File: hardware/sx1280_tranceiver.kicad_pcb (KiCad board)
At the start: 2 copper layers, 22 parts, among them J1 U.FL-R-SMT-1(80), J2 Conn_02x06_Odd_Even, U1 sx1280, U2 2450FM07D0034, Y1 ECS-520-12-37B-CTN-TR

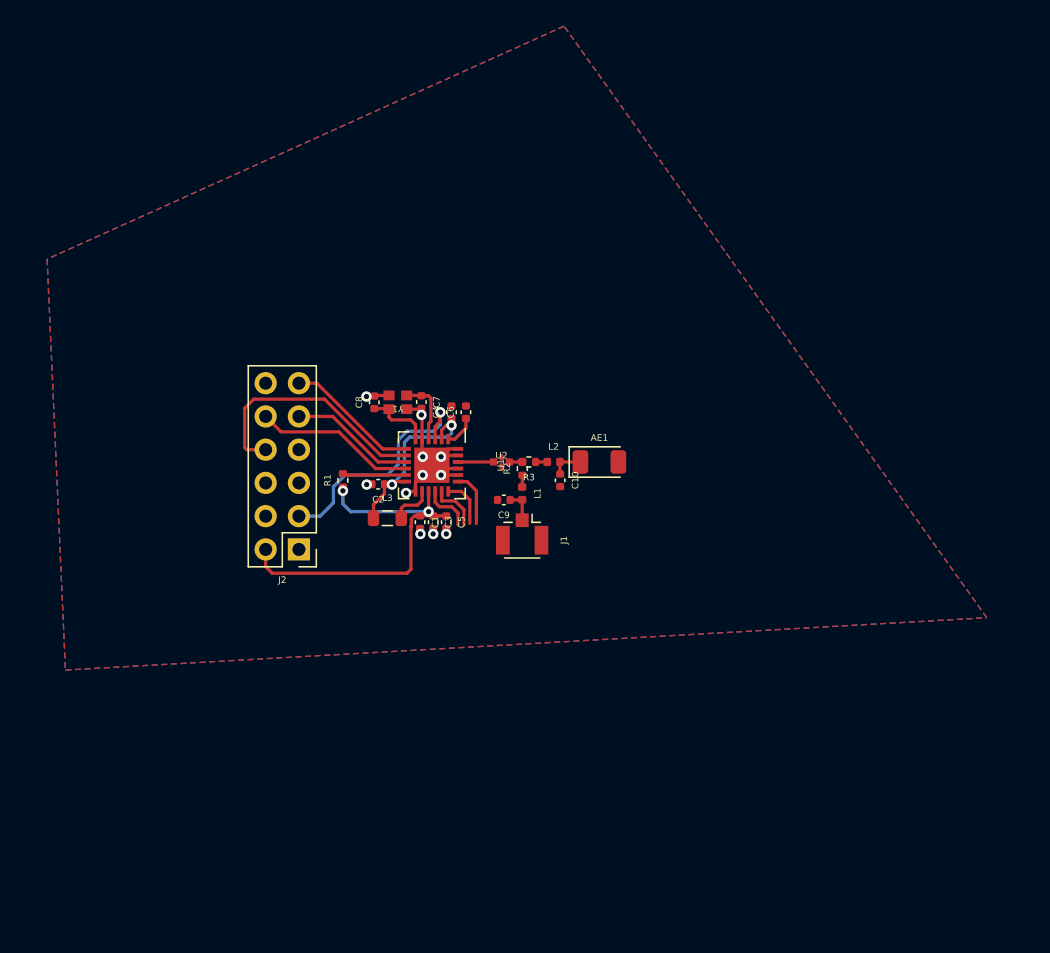
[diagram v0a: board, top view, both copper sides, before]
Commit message: finalized layout
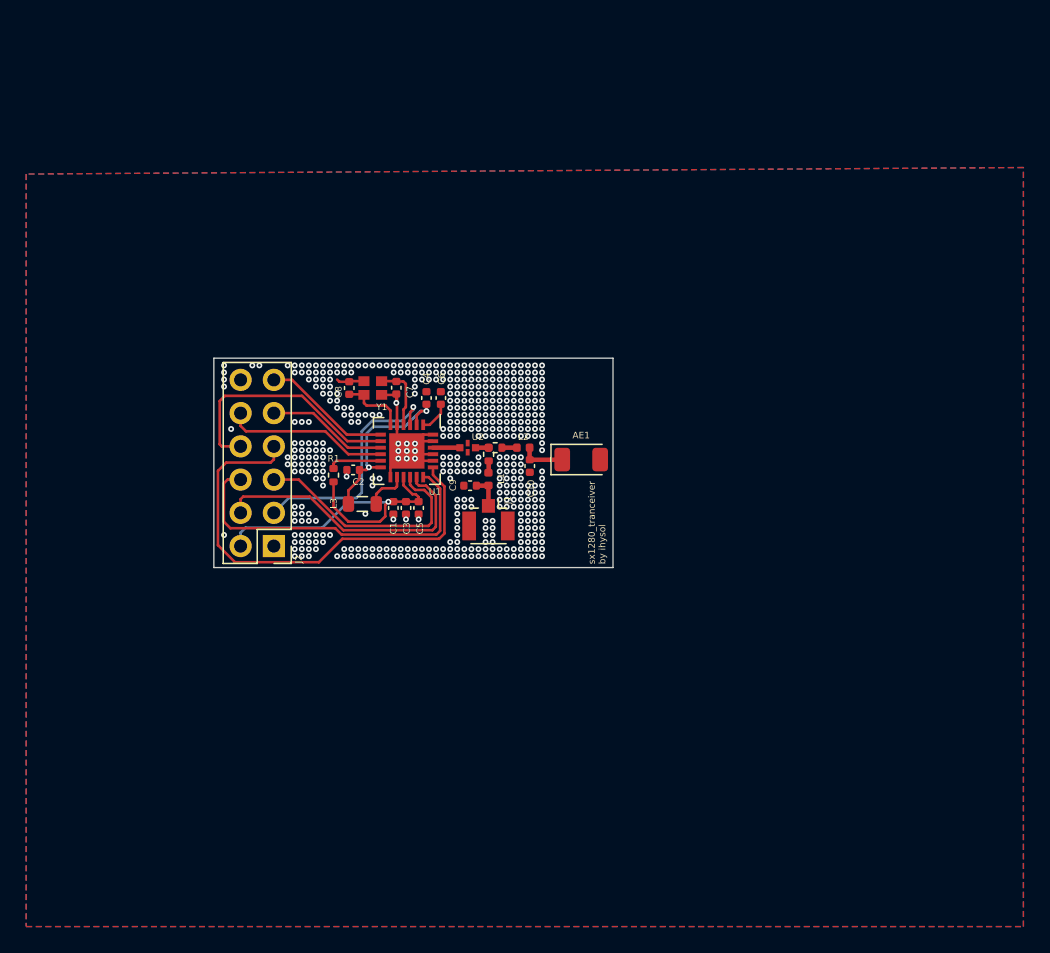
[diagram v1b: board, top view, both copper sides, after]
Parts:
- moved C9 2.80 mm to (84.7, 67.9)
- moved J1 2.80 mm to (86.1, 70.5)
- moved L1 2.80 mm to (86.1, 67.4)
- moved R2 2.80 mm to (86.1, 65.5)
- moved R3 2.80 mm to (86.6, 65.0)
- moved U2 2.80 mm to (84.5, 65.0)
- moved C10 2.56 mm to (89.3, 66.4)
- moved L2 2.56 mm to (88.8, 65.0)
- moved C5 2.38 mm to (80.8, 69.6)
- moved C3 2.35 mm to (79.8, 69.6)
- moved C1 2.32 mm to (78.9, 69.6)
- moved L3 2.20 mm to (76.5, 69.3)
- moved C7 2.20 mm to (79.1, 60.4)
- moved C8 2.20 mm to (75.5, 60.4)
- moved Y1 2.20 mm to (77.3, 60.4)
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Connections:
- J2 pad 12: ANT_SW -> unconnected-(J2-Pin_12-Pad12)
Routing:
- net SX_NSS: track 4.19 -> 35.5 mm
- net SX_SCK: track 3.72 -> 26.3 mm
- net SX_MOSI: track 3.84 -> 21.9 mm
- net SX_MISO: track 3.82 -> 18.2 mm
- net VBAT: track 29.2 -> 26.0 mm, vias 2 -> 1
- net Net-(AE1-FEED): track 2.49 -> 3.50 mm
- net VBAT_IO: track 4.85 -> 4.07 mm
- net Net-(U1-RFIO): track 2.72 -> 2.05 mm
- net GND: track 16.9 -> 16.7 mm, vias 11 -> 475
- added copper zone on In1.Cu, net GND
- added copper zone on In2.Cu, net GND
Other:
- board outline added: 30.5 x 16 mm
- copper layers 2 -> 4
- board text added: "sx1280_tranceiver by ihysol"
